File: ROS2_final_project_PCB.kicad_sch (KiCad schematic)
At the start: 18 parts, among them J1 Conn_01x03_Socket, J10 Conn_01x04_Pin, J2 Conn_01x03_Socket, J3 Motor1, J4 Motor2, J5 Motor3, J6 Motor4, J7 Conn_01x04_Pin, J8 Conn_01x04_Pin, J9 Conn_01x04_Pin, U3 ROB-14450, U4 ESP32-DevKitC, U5 ROB-14450

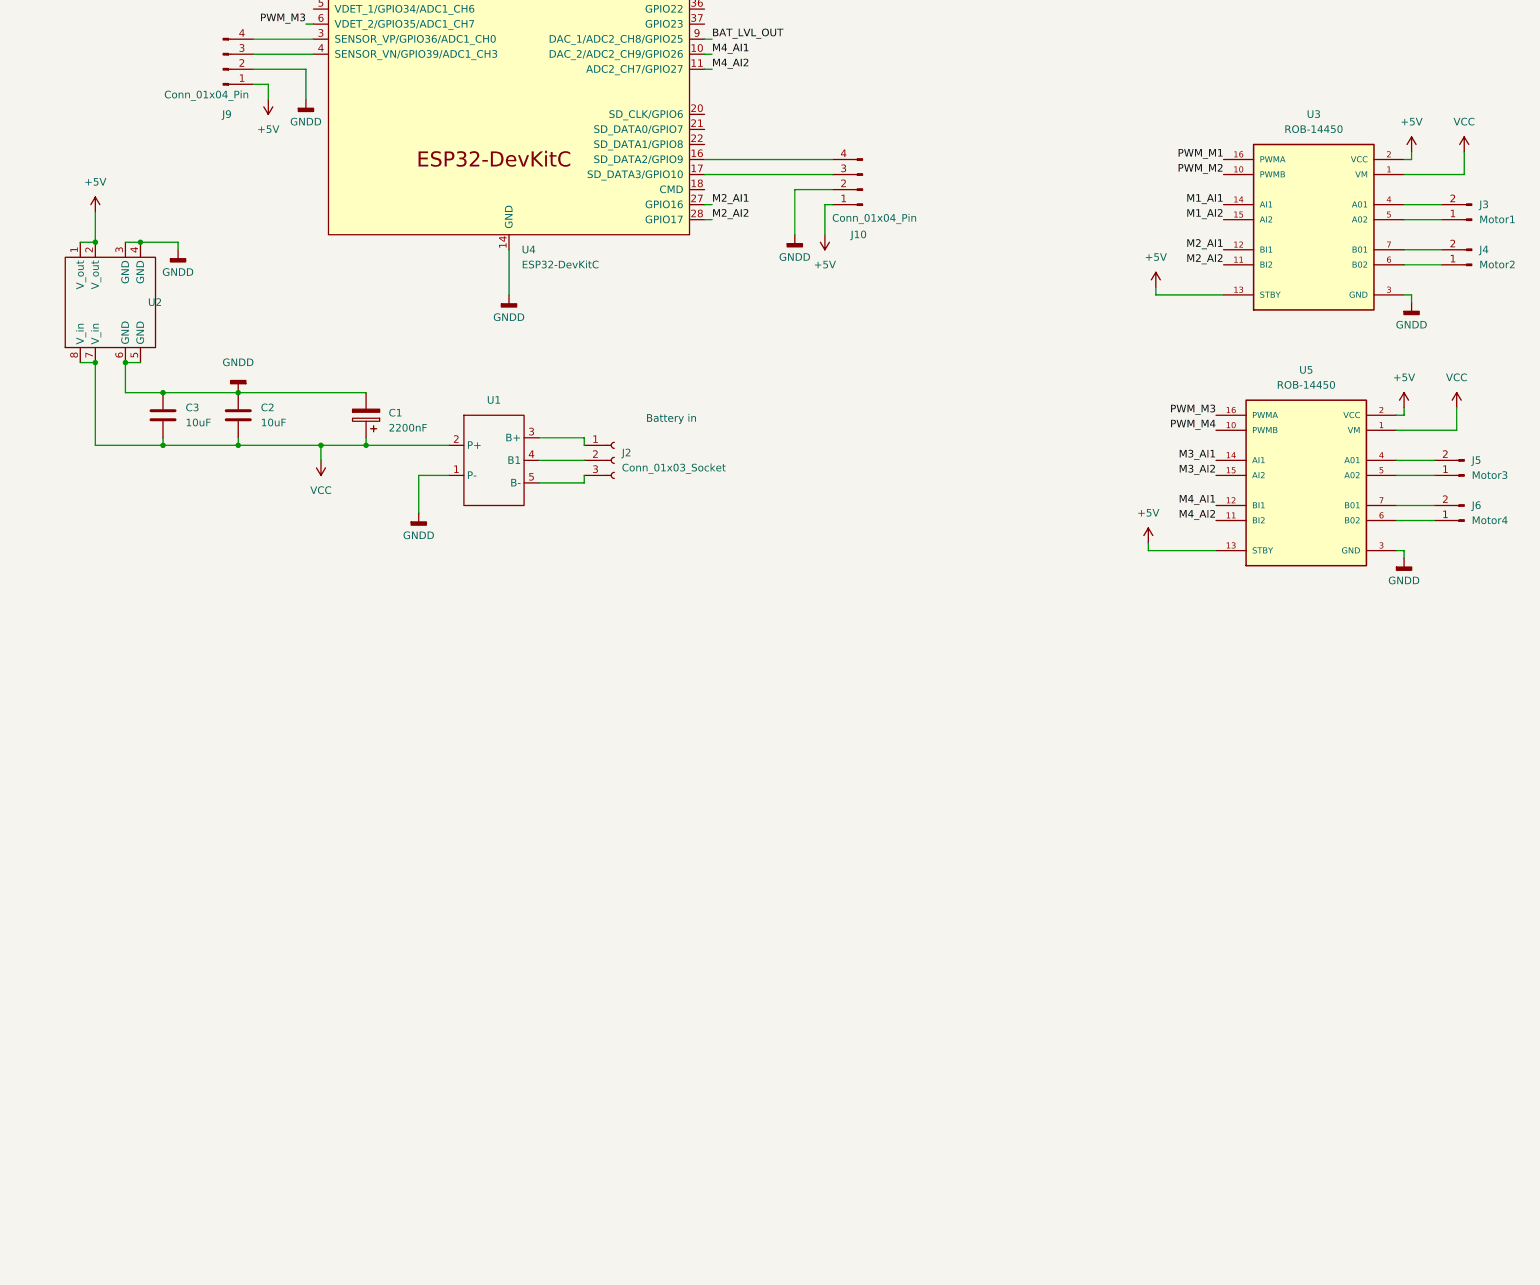
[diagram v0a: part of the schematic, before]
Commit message: ее
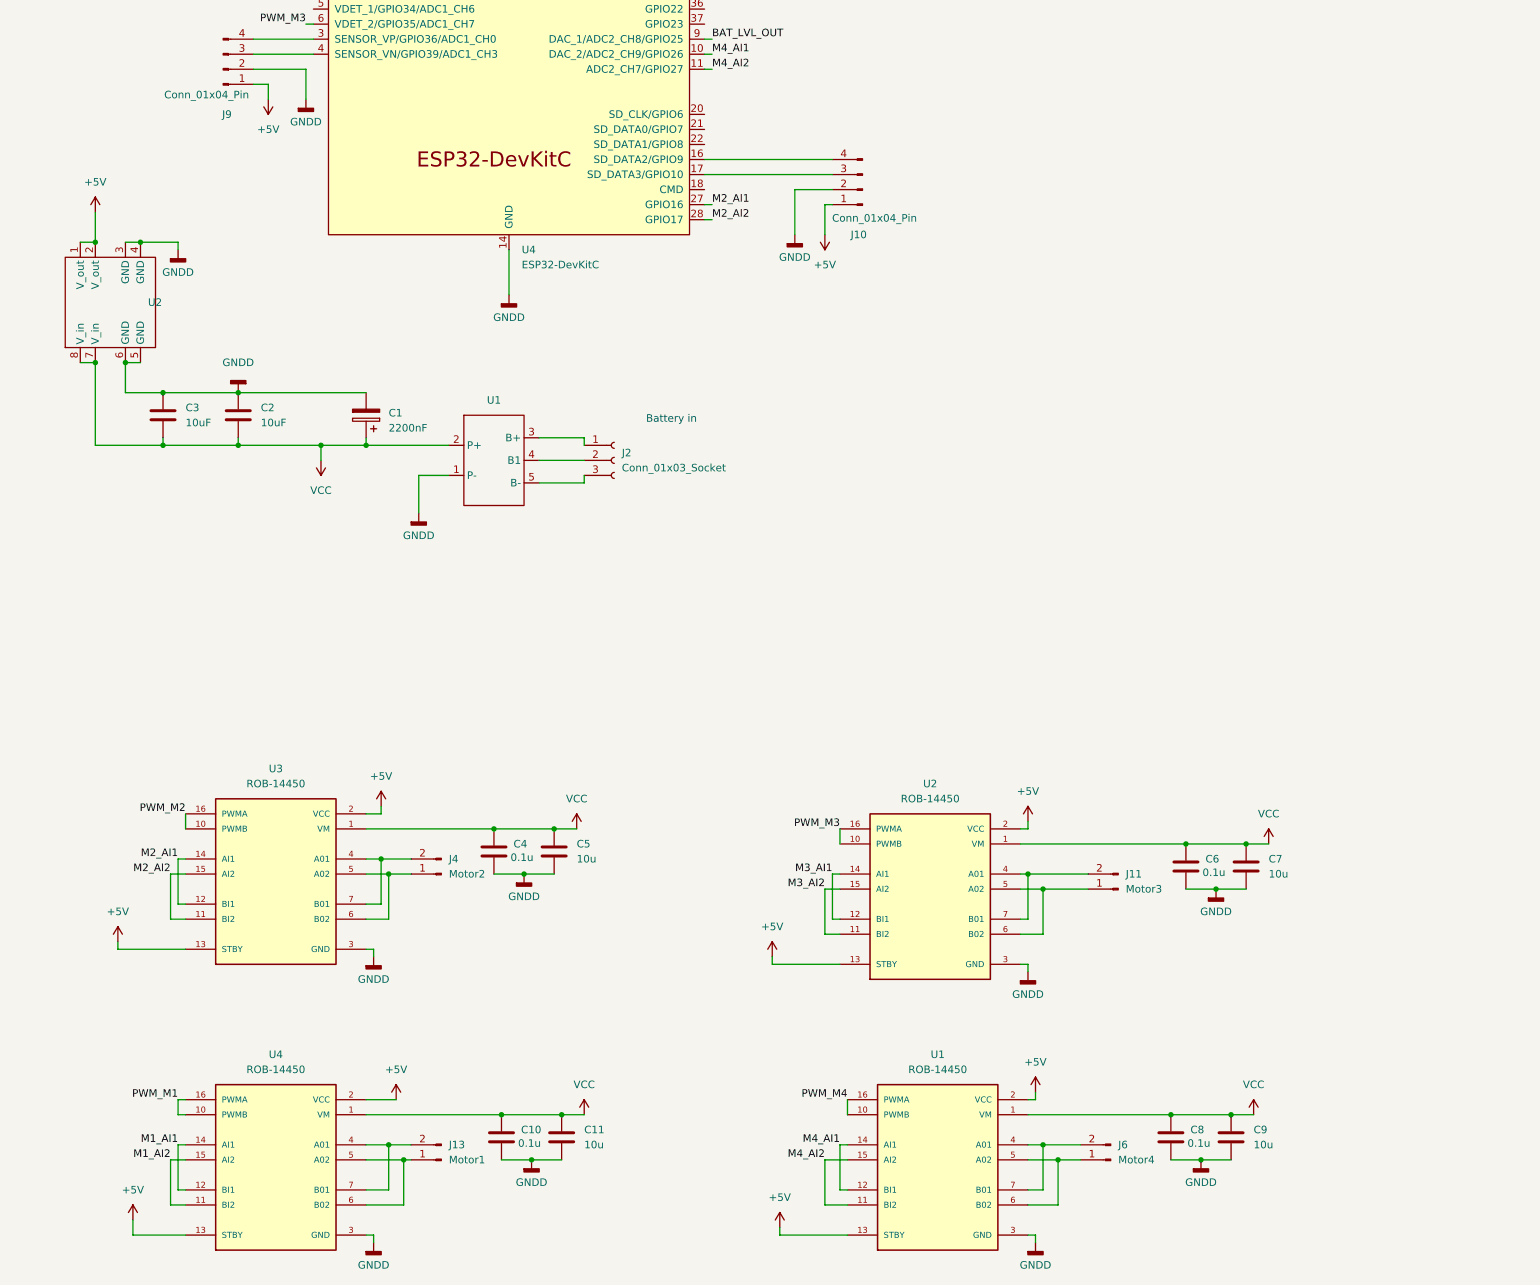
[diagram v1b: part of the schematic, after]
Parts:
- removed J3: Motor1, Connector_Molex:Molex_KK-254_AE-6410-02A_1x02_P2.54mm_Vertical, symbol Connector:Conn_01x02_Pin
- removed J5: Motor3, Connector_Molex:Molex_KK-254_AE-6410-02A_1x02_P2.54mm_Vertical, symbol Connector:Conn_01x02_Pin
- added C10, C4, C6, C8: 0.1u, symbol Device:C
- added C11, C5, C7, C9: 10u, symbol Device:C
- added J11: Motor3, Connector_Molex:Molex_KK-254_AE-6410-02A_1x02_P2.54mm_Vertical, symbol Connector:Conn_01x02_Pin
- added J13: Motor1, Connector_Molex:Molex_KK-254_AE-6410-02A_1x02_P2.54mm_Vertical, symbol Connector:Conn_01x02_Pin
- added U2, U4: ROB-14450, ROB-14450:MODULE_ROB-14450, symbol ROB-14450:ROB-14450
- renumbered U3 to U1, U5 to U3
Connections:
- net +5V: now also U2.13 (STBY), U2.2 (VCC), U4.13 (STBY), U4.2 (VCC)
- net GND: now also C10.2, C11.2, C4.2, C5.2, C6.2, C7.2, C8.2, C9.2, U2.3 (GND), U2.8 (GND), U2.9 (GND), U4.3 (GND), U4.8 (GND), U4.9 (GND)
- net M1_AI1: now also U4.12 (BI1), U4.14 (AI1); no longer U1.14 (AI1)
- net M1_AI2: now also U4.11 (BI2), U4.15 (AI2); no longer U1.15 (AI2)
- net M2_AI1: now also U3.12 (BI1), U3.14 (AI1); no longer U1.12 (BI1)
- net M2_AI2: now also U3.11 (BI2), U3.15 (AI2); no longer U1.11 (BI2)
- net M3_AI1: now also U2.12 (BI1), U2.14 (AI1); no longer U3.14 (AI1)
- net M3_AI2: now also U2.11 (BI2), U2.15 (AI2); no longer U3.15 (AI2)
- net M4_AI1: now also U1.12 (BI1), U1.14 (AI1); no longer U3.12 (BI1)
- net M4_AI2: now also U1.11 (BI2), U1.15 (AI2); no longer U3.11 (BI2)
- net PWM_M1: now also U4.10 (PWMB), U4.16 (PWMA); no longer U1.16 (PWMA)
- net PWM_M2: now also U3.10 (PWMB), U3.16 (PWMA); no longer U1.10 (PWMB)
- net PWM_M3: now also U2.10 (PWMB), U2.16 (PWMA); no longer U3.16 (PWMA)
- net PWM_M4: now also U1.10 (PWMB), U1.16 (PWMA); no longer U3.10 (PWMB)
- net VCC: now also C10.1, C11.1, C4.1, C5.1, C6.1, C7.1, C8.1, C9.1, U2.1 (VM), U4.1 (VM)
- net at J6.1 (Pin_1): now also U1.5 (A02), U1.6 (B02); no longer U3.6 (B02)
- net at J6.2 (Pin_2): now also U1.4 (A01), U1.7 (B01); no longer U3.7 (B01)
- net at J4.1 (Pin_1): now also U3.5 (A02), U3.6 (B02); no longer U1.6 (B02)
- net at J4.2 (Pin_2): now also U3.4 (A01), U3.7 (B01); no longer U1.7 (B01)
- new net: J13.1 (Pin_1), U4.5 (A02), U4.6 (B02)
- new net: J13.2 (Pin_2), U4.4 (A01), U4.7 (B01)
- new net: J11.1 (Pin_1), U2.5 (A02), U2.6 (B02)
- new net: J11.2 (Pin_2), U2.4 (A01), U2.7 (B01)
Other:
- moved on the sheet: J4, J6, U1, U3

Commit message: майже готова PCB
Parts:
- removed C10, C4, C6, C8: 0.1u, symbol Device:C
- removed J7: Conn_01x04_Pin, Connector_JST:JST_PH_B4B-PH-K_1x04_P2.00mm_Vertical, symbol Connector:Conn_01x04_Pin
- removed U2, U4: ROB-14450, ROB-14450:MODULE_ROB-14450, symbol ROB-14450:ROB-14450
- added C4, C5, C8, C9: 220uF, Capacitor_THT:CP_Radial_D13.0mm_P5.00mm, symbol Device:C_Polarized
- added D1: LED, LED_THT:LED_D3.0mm, symbol Device:LED
- added J11: switch, Connector_Molex:Molex_KK-254_AE-6410-02A_1x02_P2.54mm_Vertical, symbol Connector:Conn_01x02_Pin
- added J4: Conn_01x04_Pin, Connector_JST:JST_PH_B4B-PH-K_1x04_P2.00mm_Vertical, symbol Connector:Conn_01x04_Pin
- added R1: 560R, Resistor_THT:R_Axial_DIN0204_L3.6mm_D1.6mm_P7.62mm_Horizontal, symbol Device:R
- added U4: ZC323900, ZC323900:MODULE_ZC323900, symbol ZC323900:ZC323900
- added U8, U9: ROB-14450, ROB-14450:MODULE_ROB-14450, symbol ROB-14450:ROB-14450
- C1: renamed from C3; footprint Capacitor_THT:C_Disc_D8.0mm_W5.0mm_P7.50mm -> Capacitor_THT:C_Disc_D3.0mm_W1.6mm_P2.50mm
- C10: renamed from C5; value 10u -> 20u; footprint (none) -> Capacitor_THT:C_Disc_D4.3mm_W1.9mm_P5.00mm
- C11: renamed from C7; value 10u -> 20u; footprint (none) -> Capacitor_THT:C_Disc_D4.3mm_W1.9mm_P5.00mm
- C2: footprint Capacitor_THT:C_Disc_D8.0mm_W5.0mm_P7.50mm -> Capacitor_THT:C_Disc_D3.0mm_W1.6mm_P2.50mm
- C6: renamed from C11; value 10u -> 20u; footprint (none) -> Capacitor_THT:C_Disc_D4.3mm_W1.9mm_P5.00mm
- C7: renamed from C9; value 10u -> 20u; footprint (none) -> Capacitor_THT:C_Disc_D4.3mm_W1.9mm_P5.00mm
- U1: footprint BMS ROS2 project:Untitled -> BMS ROS2 project:BMS ROS2 project
- U2: footprint BMS ROS2 project:Untitled -> BMS ROS2 project:Buck convertor
- renumbered C1 to C3, J8 to J1, J11 to J10, J9 to J2, J2 to J3, J10 to J5, J1 to J6, J13 to J7, J6 to J8, J4 to J9, U4 to U3, U1 to U6, U3 to U7
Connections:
- net +5V: now also J4.1 (Pin_1), R1.1, U4.20 (VB), U8.13 (STBY), U8.2 (VCC), U9.13 (STBY), U9.2 (VCC)
- net BAT_LVL_OUT: now also U3.37 (GPIO23); no longer U3.9 (DAC_1/ADC2_CH8/GPIO25)
- net GND: now also C4.2, C5.2, C8.2, C9.2, D1.1 (K), J4.2 (Pin_2), U4.11 (GND), U8.3 (GND), U8.8 (GND), U8.9 (GND), U9.3 (GND), U9.8 (GND), U9.9 (GND)
- net M1_AI1: now also U4.19 (B1), U9.12 (BI1), U9.14 (AI1); no longer U3.25 (GPIO0/BOOT/ADC2_CH1)
- net M1_AI2: now also U4.18 (B2), U9.11 (BI2), U9.15 (AI2); no longer U3.24 (ADC2_CH2/GPIO2)
- net M2_AI1: now also U4.17 (B3); no longer U3.27 (GPIO16)
- net M2_AI2: now also U4.16 (B4); no longer U3.28 (GPIO17)
- net M3_AI1: now also U4.15 (B5), U8.12 (BI1), U8.14 (AI1); no longer U3.8 (32K_XN/GPIO33/ADC1_CH5)
- net M3_AI2: now also U4.14 (B6), U8.11 (BI2), U8.15 (AI2); no longer U3.7 (32K_XP/GPIO32/ADC1_CH4)
- net M4_AI1: now also U4.13 (B7); no longer U3.10 (DAC_2/ADC2_CH9/GPIO26)
- net M4_AI2: now also U4.12 (B8); no longer U3.11 (ADC2_CH7/GPIO27)
- net PWM_M1: now also U3.30 (GPIO18), U9.10 (PWMB), U9.16 (PWMA); no longer U3.23 (MTDO/GPIO15/ADC2_CH3)
- net PWM_M2: now also U3.31 (GPIO19); no longer U3.29 (GPIO5)
- net PWM_M3: now also U3.33 (GPIO21), U8.10 (PWMB), U8.16 (PWMA); no longer U3.6 (VDET_2/GPIO35/ADC1_CH7)
- net PWM_M4: now also U3.36 (GPIO22); no longer U3.12 (MTMS/GPIO14/ADC2_CH6)
- net VCC: now also C4.1, C5.1, C8.1, C9.1, J11.2 (Pin_2), U8.1 (VM), U9.1 (VM); no longer U1.2 (P+)
- net at J7.1 (Pin_1): now also U9.5 (A02), U9.6 (B02)
- net at J7.2 (Pin_2): now also U9.4 (A01), U9.7 (B01)
- net at J10.1 (Pin_1): now also U8.5 (A02), U8.6 (B02)
- net at J10.2 (Pin_2): now also U8.4 (A01), U8.7 (B01)
- net +3.3V: now reaches U3.1 (3V3)
- net +3.3V: now also U4.1 (VA), U4.10 (OE)
- net M4_AI2_3.3: now reaches U3.20 (SD_CLK/GPIO6)
- net M4_AI2_3.3: now also U4.9 (A8)
- net M4_AI1_3.3: now reaches U3.21 (SD_DATA0/GPIO7)
- net M4_AI1_3.3: now also U4.8 (A7)
- net M3_AI2_3.3: now reaches U3.22 (SD_DATA1/GPIO8)
- net M3_AI2_3.3: now also U4.7 (A6)
- net M1_AI2_3.3: now reaches U3.26 (ADC2_CH0/GPIO4)
- net M1_AI2_3.3: now also U4.3 (A2)
- new net: D1.2 (A), R1.2
- new net: J11.1 (Pin_1), U1.2 (P+)
- new net: J4.3 (Pin_3), U3.7 (32K_XP/GPIO32/ADC1_CH4)
- new net: J4.4 (Pin_4), U3.8 (32K_XN/GPIO33/ADC1_CH5)
- new net M1_AI1_3.3: U3.27 (GPIO16), U4.2 (A1)
- new net M2_AI1_3.3: U3.25 (GPIO0/BOOT/ADC2_CH1), U4.4 (A3)
- new net M2_AI2_3.3: U3.24 (ADC2_CH2/GPIO2), U4.5 (A4)
- new net M3_AI1_3.3: U3.23 (MTDO/GPIO15/ADC2_CH3), U4.6 (A5)
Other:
- moved on the sheet: C1, C10, C11, C2, C3, C6, C7, J1, J10, J2, J3, J5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
